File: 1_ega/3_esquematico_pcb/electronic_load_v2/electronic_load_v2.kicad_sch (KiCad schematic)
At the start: 67 parts, among them J1 Encoder, J11 LOAD, J12 Memoria SD, J13 LCD, J15 VCC, J16 RTC, J17 EGB, J3 GND, J6 RPico PWR, J7 GND, J8 5V, Q1 IRF540N, Q3 BC327, Q4 BC327, SW1 BTN_MENU, SW2 BTN_STOP, SW3 SW_PWR, U1 LM324, U2 INA219AxD, U3 LM7805_TO220

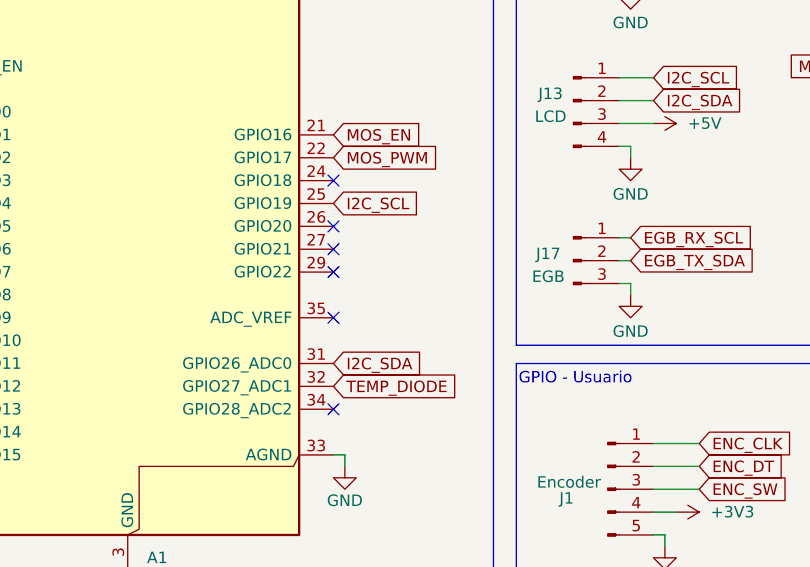
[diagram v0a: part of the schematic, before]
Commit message: chore: add name and logo
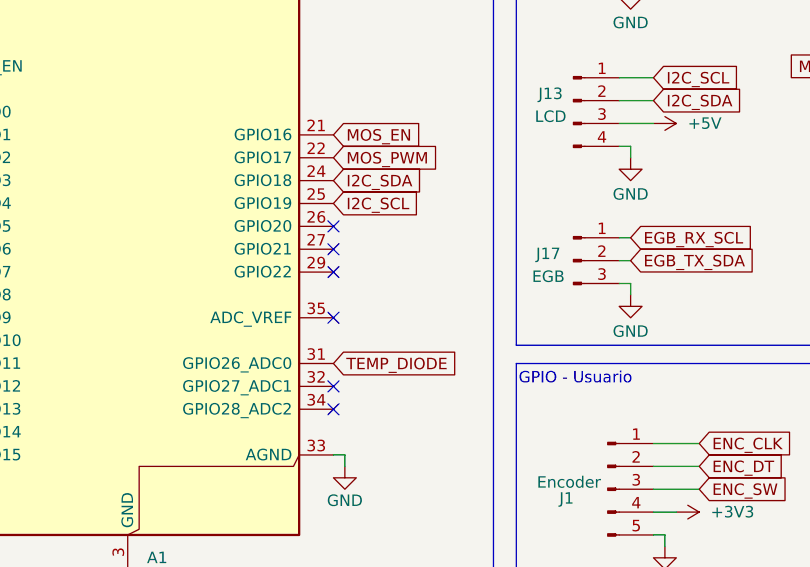
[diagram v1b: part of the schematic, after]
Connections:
- net I2C_SDA: now also A1.24 (GPIO18); no longer A1.31 (GPIO26_ADC0)
- net TEMP_DIODE: now also A1.31 (GPIO26_ADC0); no longer A1.32 (GPIO27_ADC1)
